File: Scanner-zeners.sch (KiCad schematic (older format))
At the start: 44 parts, among them J1 Conn_01x04, J2 Battery connector, Q1 BC548, Q2 BC548, Q3 BC548, Q4 BC548, Q5 BC548, Q6 BC548, U1 S4EBL25V, U2 S4EBL25V, U3 PC817, U4 PC817, U5 PC817, U6 4028, U7 S4EBL25V, U8 S4EBL25V

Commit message: Modifiqué el esquemático para tener más pines.
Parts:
- removed J1: Conn_01x04, Pin_Headers:Pin_Header_Straight_1x04_Pitch2.54mm, symbol Scanner-zeners-rescue:Conn_01x04
- added J1: Conn_01x20_Male, Connector_PinHeader_2.54mm:PinHeader_1x20_P2.54mm_Horizontal, symbol Connector:Conn_01x20_Male
- added J3: Battery connector, Pin_Headers:Pin_Header_Straight_2x01_Pitch2.54mm, symbol Scanner-zeners-rescue:Conn_01x02
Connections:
- wire segments 103 -> 105
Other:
- moved on the sheet: R11, R12, R13, R5, R6, R7, U3, U4, U5, U6

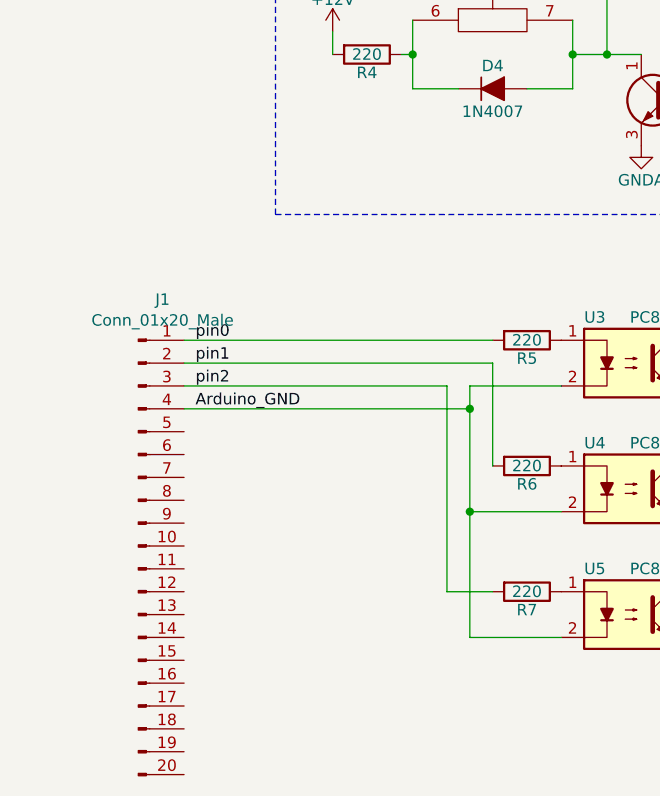
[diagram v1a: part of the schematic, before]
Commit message: Version para back panel lista
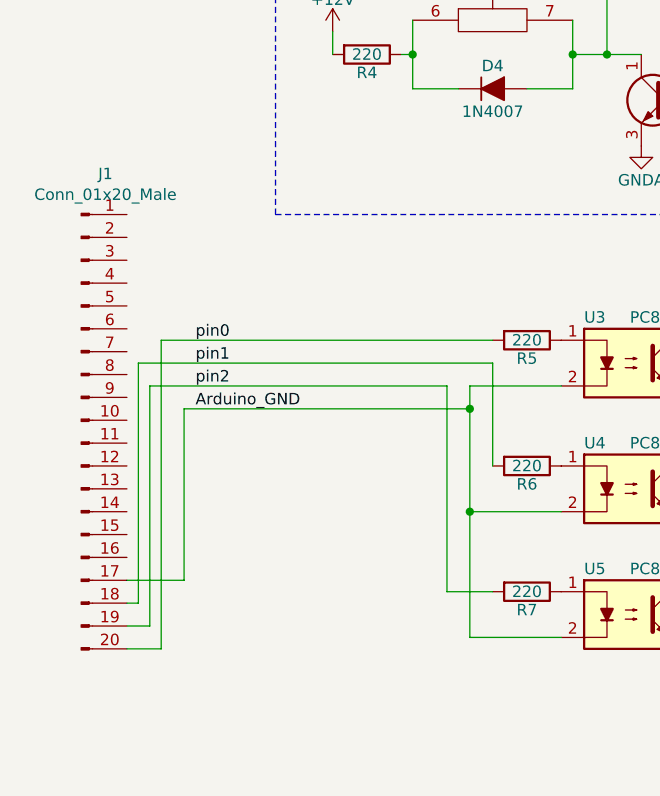
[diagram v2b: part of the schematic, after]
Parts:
- J2, J3: footprint Pin_Headers:Pin_Header_Straight_2x01_Pitch2.54mm -> Connector_PinHeader_2.54mm:PinHeader_1x02_P2.54mm_Vertical
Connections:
- net Arduino_GND: now also J1.17 (Pin_17); no longer J1.4 (Pin_4)
- net pin0: now also J1.20 (Pin_20); no longer J1.1 (Pin_1)
- net pin1: now also J1.18 (Pin_18); no longer J1.2 (Pin_2)
- net pin2: now also J1.19 (Pin_19); no longer J1.3 (Pin_3)
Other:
- moved on the sheet: J1
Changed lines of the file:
@@
 F 0 "J2" H 7150 6050 50  0000 C CNN
 F 1 "Battery connector" H 7150 5750 50  0000 C CNN
-F 2 "Pin_Headers:Pin_Header_Straight_2x01_Pitch2.54mm" H 7150 5950 50  0001 C CNN
+F 2 "Connector_PinHeader_2.54mm:PinHeader_1x02_P2.54mm_Vertical" H 7150 5950 50  0001 C CNN
 F 3 "" H 7150 5950 50  0001 C CNN
 	1    7150 5950
@@
 Wire Wire Line
 	1450 6000 2700 6000
-Wire Wire Line
-	1450 5900 2600 5900
-Wire Wire Line
-	1450 5800 2800 5800
-Wire Wire Line
-	1450 5700 2800 5700
 Text Label 1500 6000 0    50   ~ 0
 Arduino_GND
@@
 L Connector:Conn_01x20_Male J1
 U 1 1 5CE5B250
-P 1250 6600
-F 0 "J1" H 1356 7678 50  0000 C CNN
-F 1 "Conn_01x20_Male" H 1356 7587 50  0000 C CNN
-F 2 "Connector_PinHeader_2.54mm:PinHeader_1x20_P2.54mm_Horizontal" H 1250 6600 50  0001 C CNN
-F 3 "~" H 1250 6600 50  0001 C CNN
-	1    1250 6600
+P 1000 6050
+F 0 "J1" H 1106 7128 50  0000 C CNN
+F 1 "Conn_01x20_Male" H 1106 7037 50  0000 C CNN
+F 2 "Connector_PinHeader_2.54mm:PinHeader_1x20_P2.54mm_Horizontal" H 1000 6050 50  0001 C CNN
+F 3 "~" H 1000 6050 50  0001 C CNN
+	1    1000 6050
 	1    0    0    -1
 $EndComp
@@
 F 0 "J3" H 7550 6050 50  0000 C CNN
 F 1 "Battery connector" H 7550 5750 50  0000 C CNN
-F 2 "Pin_Headers:Pin_Header_Straight_2x01_Pitch2.54mm" H 7550 5950 50  0001 C CNN
+F 2 "Connector_PinHeader_2.54mm:PinHeader_1x02_P2.54mm_Vertical" H 7550 5950 50  0001 C CNN
 F 3 "" H 7550 5950 50  0001 C CNN
 	1    7550 5950
@@
 Wire Wire Line
 	6950 6050 7350 6050
+Wire Wire Line
+	1350 5700 1350 7050
+Wire Wire Line
+	1350 7050 1200 7050
+Wire Wire Line
+	1350 5700 2800 5700
+Wire Wire Line
+	1300 5900 1300 6950
+Wire Wire Line
+	1300 6950 1200 6950
+Wire Wire Line
+	1300 5900 2600 5900
+Wire Wire Line
+	1250 5800 1250 6850
+Wire Wire Line
+	1250 6850 1200 6850
+Wire Wire Line
+	1250 5800 2800 5800
+Wire Wire Line
+	1450 6000 1450 6750
+Wire Wire Line
+	1450 6750 1200 6750
 $EndSCHEMATC
